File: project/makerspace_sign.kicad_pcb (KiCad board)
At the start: 2 copper layers, 76.2 x 98 mm, 23 parts, among them J1 Conn_EXT, J2 Conn_E1_M, J3 Conn_E1_F, J4 Conn_OTH_M, J5 Conn_OTH_F, J6 Conn_E2_F, J7 Conn_E2_M

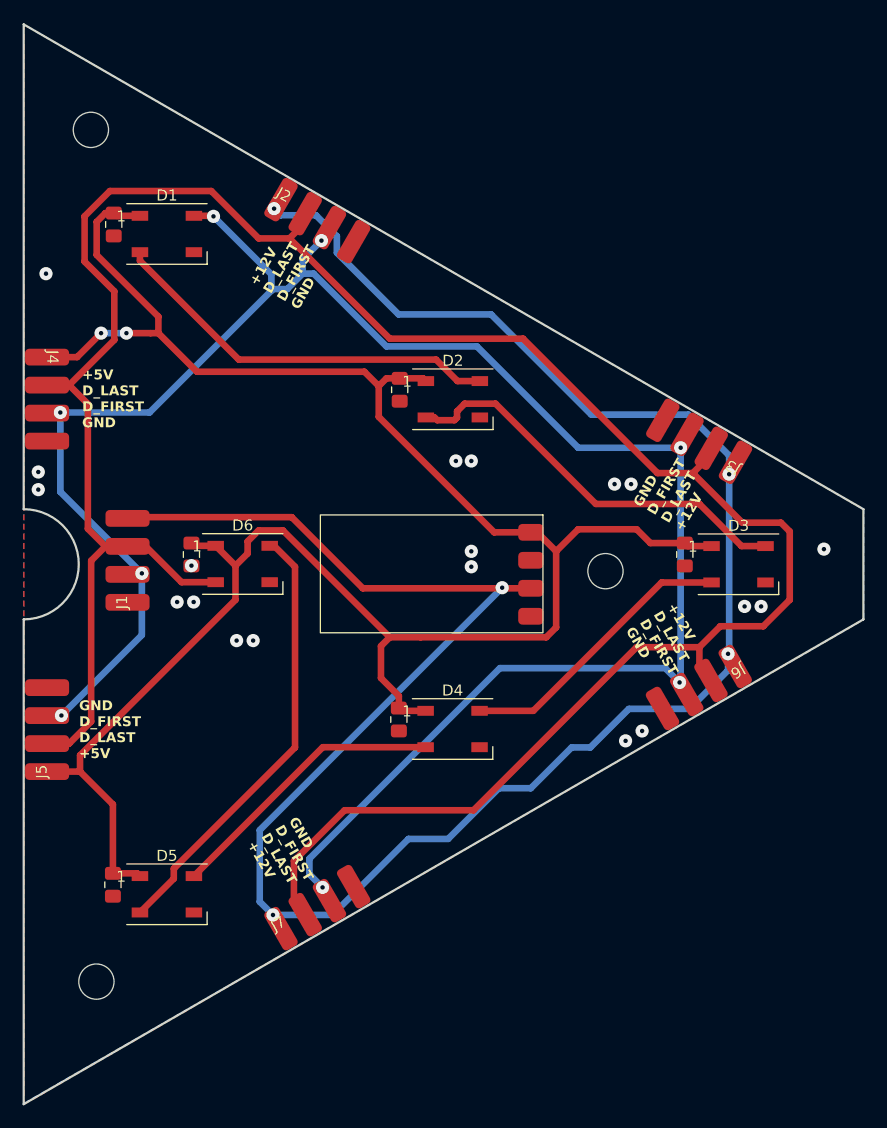
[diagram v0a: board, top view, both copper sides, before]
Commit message: v2
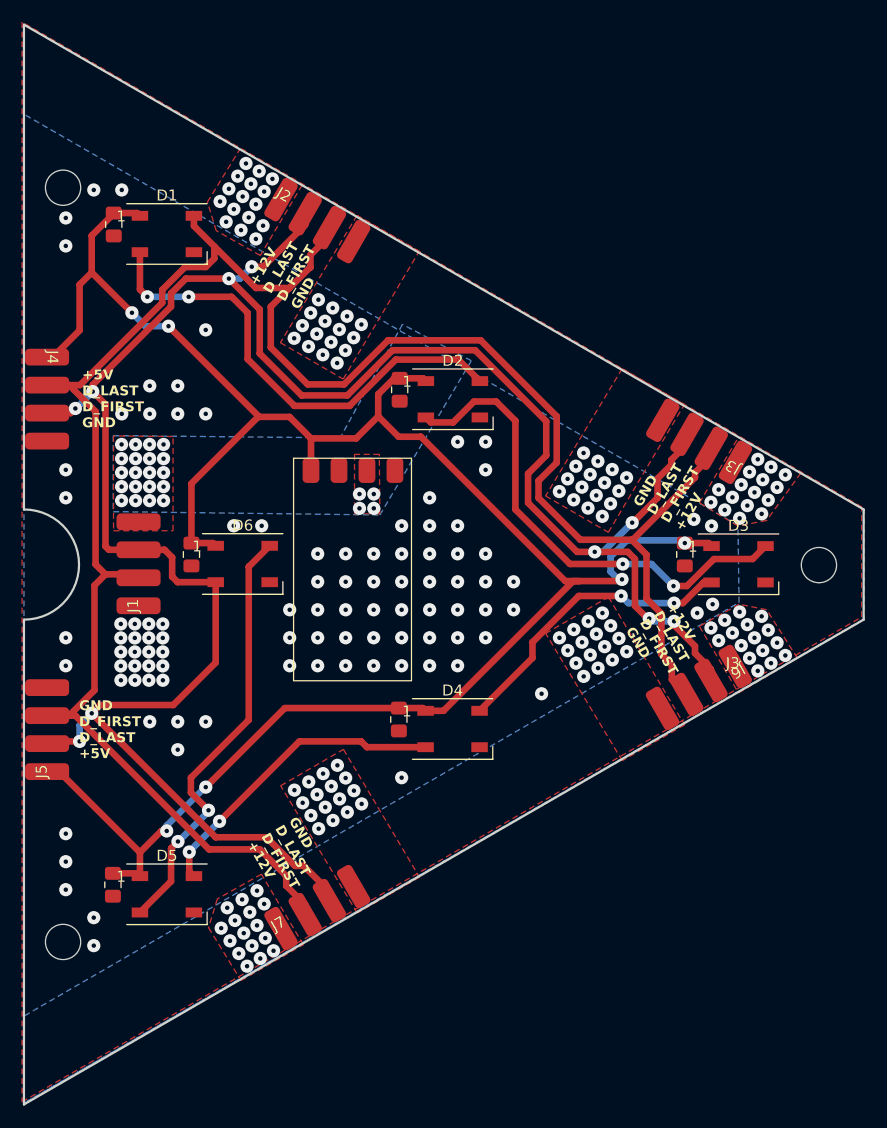
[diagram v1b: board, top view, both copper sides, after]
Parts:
- moved Buck1 23.2 mm to (86.5, 85.8), turned to 0 degrees
- moved H2 19.4 mm to (134.2, 95.5)
- moved H1 5.83 mm to (65.5, 61.2)
- moved H3 4.70 mm to (65.5, 129.7)
- moved J1 1.05 mm to (72.4, 99.1)
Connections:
- J3 pad 2: /D_LAST -> /D_FIRST
- J3 pad 3: /D_FIRST -> /D_LAST
- J4 pad 2: /D_LAST -> /D_FIRST
- J4 pad 3: /D_FIRST -> /D_LAST
- J7 pad 2: /D_LAST -> /D_FIRST
- J7 pad 3: /D_FIRST -> /D_LAST
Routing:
- net +12V: track 200.2 -> 0.00 mm, vias 5 -> 88
- net /D_LAST: track 222.0 -> 204.6 mm, vias 0 -> 10
- net /D_FIRST: track 182.0 -> 194.8 mm, vias 8 -> 0
- net /D_23: track 37.2 -> 45.0 mm, vias 0 -> 2
- net /D_12: track 36.2 -> 43.6 mm, vias 0 -> 2
- net +5V: track 191.7 -> 185.5 mm, vias 2 -> 6
- net /D_45: track 25.9 -> 28.2 mm, vias 0 -> 2
- net /D_34: track 25.9 -> 27.2 mm, vias 0 -> 2
- net /D_56: track 40.3 -> 39.5 mm, vias 0 -> 2
- net GND: vias 19 -> 162
- added copper zone on B.Cu, net +12V
- added copper zone on F.Cu, net +12V
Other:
- board text added: "GND D_LAST D_FIRST +12V"
- board text added: "J3"
- board text removed: "GND D_FIRST D_LAST +12V"
